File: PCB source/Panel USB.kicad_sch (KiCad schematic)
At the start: 9 parts, among them J5 Connector, USB-TYPE-C-16P, U1 PESD5V0S2BT

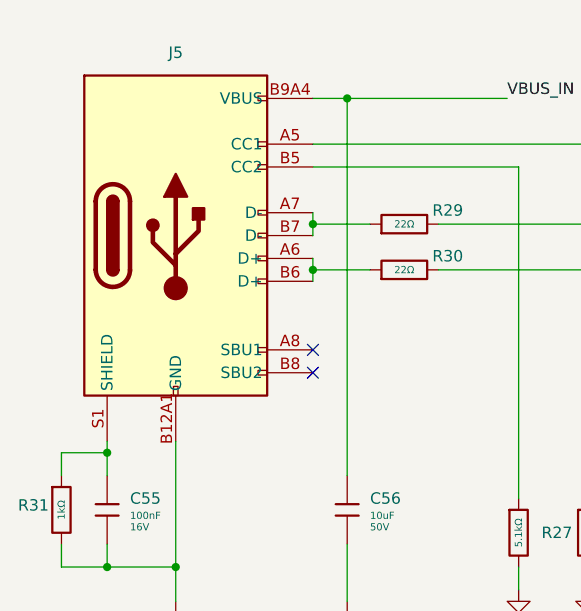
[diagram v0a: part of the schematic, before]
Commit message: Finish layout
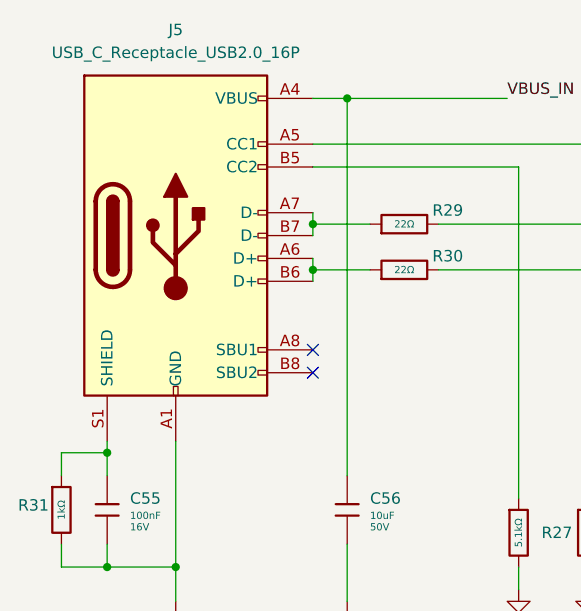
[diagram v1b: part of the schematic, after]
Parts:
- removed J5: Connector, USB-TYPE-C-16P, Connector_USB:USB_C_Receptacle_GCT_USB4105-xx-A_16P_TopMnt_Horizontal, symbol PCM_JLCPCB-Extended:Connector, USB-TYPE-C-16P
- added J5: USB_C_Receptacle_USB2.0_16P, Connector_USB:USB_C_Receptacle_GCT_USB4105-xx-A_16P_TopMnt_Horizontal, symbol Connector:USB_C_Receptacle_USB2.0_16P
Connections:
- net GND: now also J5.A1 (GND), J5.A12 (GND), J5.B1 (GND), J5.B12 (GND)
- net VBUS_IN: now also J5.A4 (VBUS), J5.A9 (VBUS), J5.B4 (VBUS), J5.B9 (VBUS)
- net at C55.1, R31.1: now also J5.S1 (SHIELD)
- net at R29.1: now also J5.A7 (D-), J5.B7 (D-)
- net at R28.1: now also J5.A5 (CC1)
- net at R30.1: now also J5.A6 (D+), J5.B6 (D+)
- net at R27.1: now also J5.B5 (CC2)
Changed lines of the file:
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@@
-	)
-	(symbol
-		(lib_id "PCM_JLCPCB-Extended:Connector, USB-TYPE-C-16P")
-		(at 96.52 85.09 0)
-		(unit 1)
-		(exclude_from_sim no)
-		(in_bom yes)
-		(on_board yes)
-		(dnp no)
-		(fields_autoplaced yes)
-		(property "Reference" "J5"
-			(at 96.52 64.77 0)
-			(effects
-				(font
-					(size 1.27 1.27)
-				)
-			)
-		)
-		(property "Value" "Connector, USB-TYPE-C-16P"
-			(at 99.06 86.36 0)
-			(effects
-				(font
-					(size 1.27 1.27)
-				)
-				(hide yes)
-			)
-		)
-		(property "Footprint" "Connector_USB:USB_C_Receptacle_GCT_USB4105-xx-A_16P_TopMnt_Horizontal"
-			(at 96.52 95.25 0)
-			(effects
-				(font
-					(size 1.27 1.27)
-					(italic yes)
-				)
-				(hide yes)
-			)
-		)
-		(property "Datasheet" "https://atta.szlcsc.com/upload/public/pdf/source/20220920/0EF8F885FCCEA71F60E9E85152155021.pdf"
-			(at 94.234 84.963 0)
-			(effects
-				(font
-					(size 1.27 1.27)
-				)
-				(justify left)
-				(hide yes)
-			)
-		)
-		(property "Description" "3A 1 Horizontal attachment 16P Female -25℃~+85℃ Type-C SMD USB Connectors ROHS"
-			(at 99.06 83.82 0)
-			(effects
-				(font
-					(size 1.27 1.27)
-				)
-				(hide yes)
-			)
-		)
-		(property "LCSC" "C2927039"
-			(at 99.06 83.82 0)
-			(effects
-				(font
-					(size 1.27 1.27)
-				)
-				(hide yes)
-			)
-		)
-		(pin "A6"
-		)
-		(pin "A12B1"
-		)
-		(pin "S1"
-		)
-		(pin "B8"
-		)
-		(pin "B12A1"
-		)
-		(pin "A9B4"
-		)
-		(pin "A7"
-		)
-		(pin "A5"
-		)
-		(pin "A8"
-		)
-		(pin "B6"
-		)
-		(pin "B7"
-		)
-		(pin "B9A4"
-		)
-		(pin "B5"
-		)
-		(instances
-			(project ""
-				(path "/3103c9de-f1ba-4d51-8bfc-798df1c75e2f/86d81324-cbad-4692-8b67-2c038a3e8215"
-					(reference "J5")
-					(unit 1)
-				)
-			)
-		)
 	)
 	(symbol
@@
 					(unit 1)
 				)
+			)
+		)
+	)
+	(symbol
+		(lib_name "USB_C_Receptacle_USB2.0_16P_1")
+		(lib_id "Connector:USB_C_Receptacle_USB2.0_16P")
+		(at 96.52 85.09 0)
+		(unit 1)
+		(exclude_from_sim no)
+		(in_bom yes)
+		(on_board yes)
+		(dnp no)
+		(fields_autoplaced yes)
+		(property "Reference" "J5"
+			(at 96.52 62.23 0)
+			(effects
+				(font
+					(size 1.27 1.27)
+				)
+			)
+		)
+		(property "Value" "USB_C_Receptacle_USB2.0_16P"
+			(at 96.52 64.77 0)
+			(effects
+				(font
+					(size 1.27 1.27)
+				)
+			)
+		)
+		(property "Footprint" "Connector_USB:USB_C_Receptacle_GCT_USB4105-xx-A_16P_TopMnt_Horizontal"
+			(at 100.33 85.09 0)
+			(effects
+				(font
+					(size 1.27 1.27)
+				)
+				(hide yes)
+			)
+		)
+		(property "Datasheet" "https://www.usb.org/sites/default/files/documents/usb_type-c.zip"
+			(at 100.33 85.09 0)
+			(effects
+				(font
+					(size 1.27 1.27)
+				)
+				(hide yes)
+			)
+		)
+		(property "Description" "USB 2.0-only 16P Type-C Receptacle connector"
+			(at 96.52 85.09 0)
+			(effects
+				(font
+					(size 1.27 1.27)
+				)
+				(hide yes)
+			)
+		)
+		(pin "A4"
+		)
+		(pin "B9"
+		)
+		(pin "A8"
+		)
+		(pin "A9"
+		)
+		(pin "B1"
+		)
+		(pin "S1"
+		)
+		(pin "A1"
+		)
+		(pin "B12"
+		)
+		(pin "A7"
+		)
+		(pin "B6"
+		)
+		(pin "B8"
+		)
+		(pin "A5"
+		)
+		(pin "A6"
+		)
+		(pin "B5"
+		)
+		(pin "B4"
+		)
+		(pin "B7"
+		)
+		(pin "A12"
+		)
+		(instances
+			(project "OrangePie"
+				(path "/3103c9de-f1ba-4d51-8bfc-798df1c75e2f/86d81324-cbad-4692-8b67-2c038a3e8215"
+					(reference "J5")
+					(unit 1)
+				)

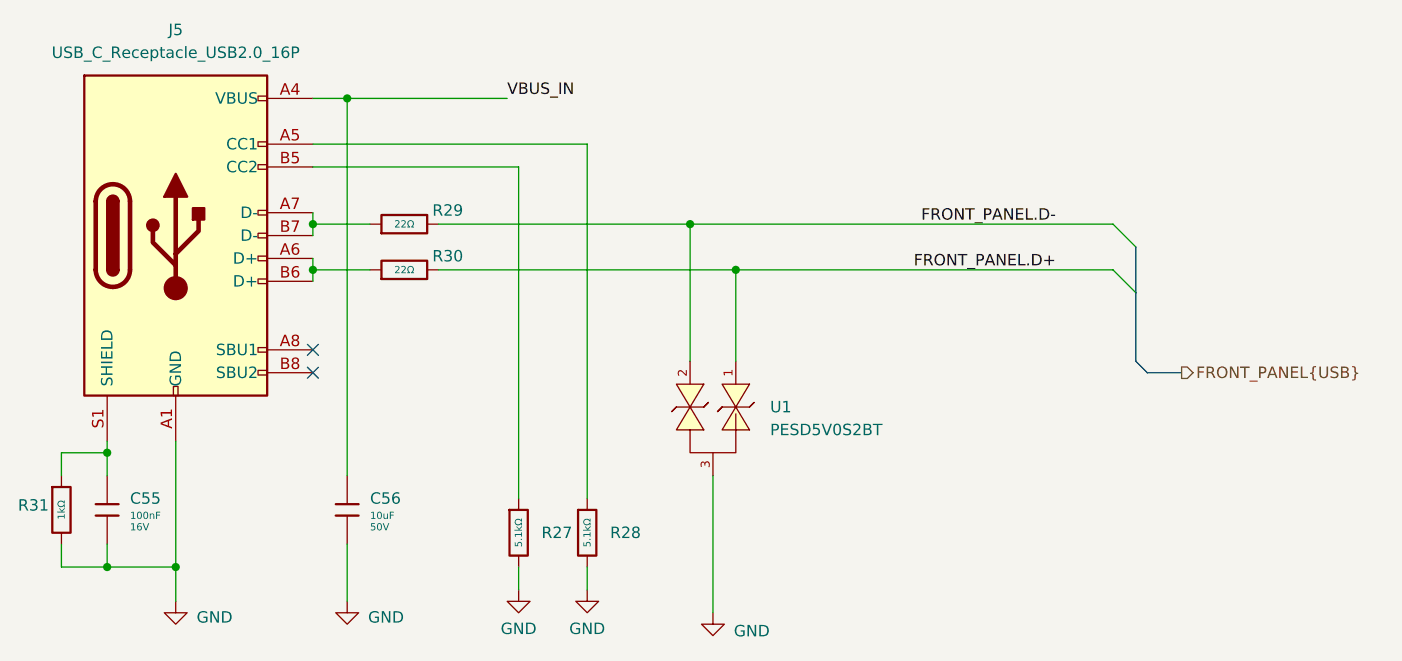
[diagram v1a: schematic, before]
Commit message: Fix schematic
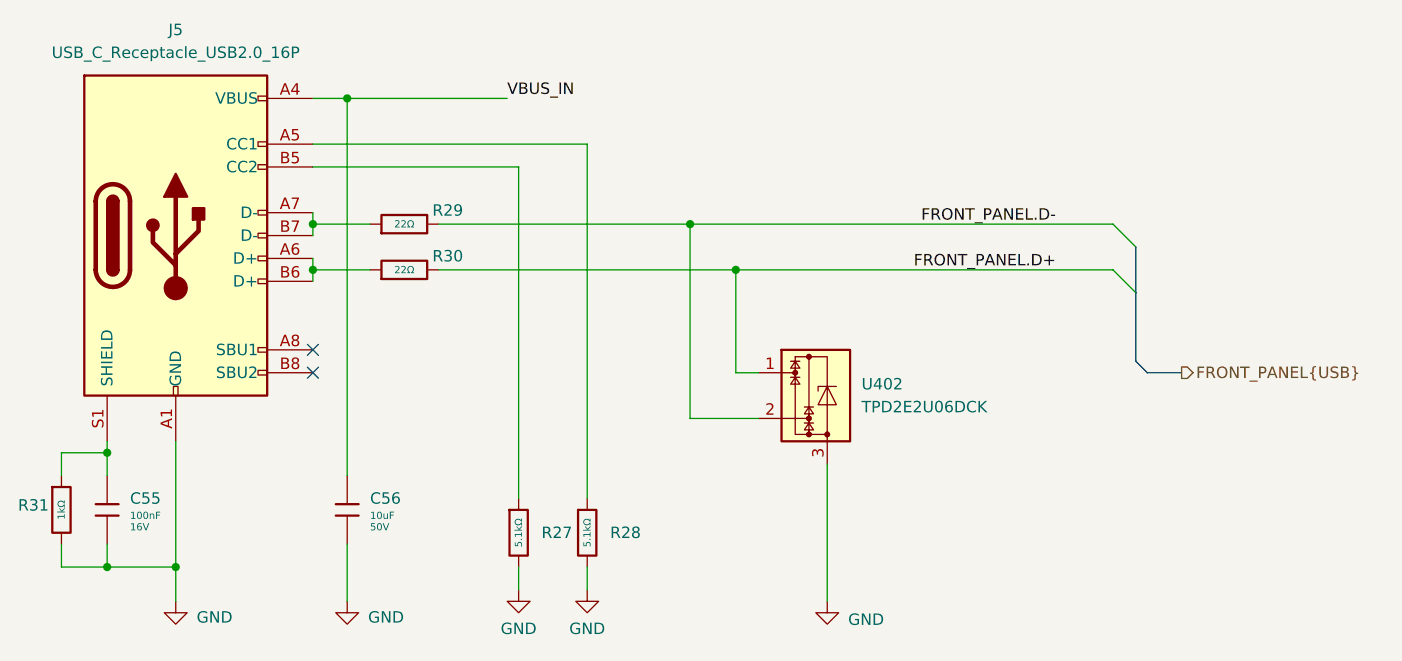
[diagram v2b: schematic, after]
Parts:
- removed U1: PESD5V0S2BT, Package_TO_SOT_SMD:SOT-23, symbol PESD5V0S2BT:PESD5V0S2BT
- added U402: TPD2E2U06DCK, Package_TO_SOT_SMD:SOT-323_SC-70, symbol Power_Protection:TPD2E2U06DCK
- C55: Stock 27771805 -> 19831671
- C56: Price 0.067USD -> 0.069USD; Stock 1423931 -> 1211974
- R27, R28: Stock 2578203 -> 3416329
- R29, R30: Stock 2497993 -> 2158519
- R31: Stock 10672962 -> 7947916
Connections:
- net FRONT_PANEL.D+: now also U402.1
- net FRONT_PANEL.D-: now also U402.2
- net GND: now also U402.3
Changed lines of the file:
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@@
 (kicad_sch
-	(version 20231120)
+	(version 20250114)
 	(generator "eeschema")
-	(generator_version "8.0")
+	(generator_version "9.0")
 	(paper "A4")
 	(title_block
@@
 		)
 	)
-	(wire
-		(pts
-			(xy 158.75 88.9) (xy 158.75 99.06)
-		)
-		(stroke
-			(width 0)
-			(type default)
-		)
-	)
-	(wire
-		(pts
-			(xy 153.67 83.82) (xy 153.67 99.06)
-		)
-		(stroke
-			(width 0)
-			(type default)
-		)
-	)
 	(bus
 		(pts
@@
 	(wire
 		(pts
+			(xy 153.67 105.41) (xy 161.29 105.41)
+		)
+		(stroke
+			(width 0)
+			(type default)
+		)
+	)
+	(wire
+		(pts
+			(xy 158.75 88.9) (xy 158.75 100.33)
+		)
+		(stroke
+			(width 0)
+			(type default)
+		)
+	)
+	(wire
+		(pts
 			(xy 111.76 88.9) (xy 111.76 90.17)
 		)
@@
 	(wire
 		(pts
-			(xy 156.21 111.76) (xy 156.21 127)
+			(xy 168.91 110.49) (xy 168.91 125.73)
 		)
 		(stroke
@@
 		(pts
 			(xy 111.76 83.82) (xy 111.76 85.09)
+		)
+		(stroke
+			(width 0)
+			(type default)
+		)
+	)
+	(wire
+		(pts
+			(xy 153.67 83.82) (xy 153.67 105.41)
+		)
+		(stroke
+			(width 0)
+			(type default)
+		)
+	)
+	(wire
+		(pts
+			(xy 158.75 100.33) (xy 161.29 100.33)
 		)
 		(stroke
@@
 	(label "FRONT_PANEL.D+"
 		(at 194.31 88.9 180)
-		(fields_autoplaced yes)
 		(effects
 			(font
@@
 	(label "FRONT_PANEL.D-"
 		(at 194.31 83.82 180)
-		(fields_autoplaced yes)
 		(effects
 			(font
@@
 	(label "VBUS_IN"
 		(at 133.35 69.85 0)
-		(fields_autoplaced yes)
 		(effects
 			(font
@@
 		(shape output)
 		(at 208.28 100.33 0)
-		(fields_autoplaced yes)
 		(effects
 			(font
@@
 			)
 		)
-		(property "Stock" "27771805"
+		(property "Stock" "19831671"
 			(at 88.9 115.57 0)
 			(effects
@@
 			)
 		)
-		(property "Stock" "2497993"
+		(property "Stock" "2158519"
 			(at 121.92 83.82 0)
 			(effects
@@
 			)
 		)
-		(property "Stock" "2578203"
+		(property "Stock" "3416329"
 			(at 142.24 118.11 0)
 			(effects
@@
 	(symbol
 		(lib_id "power:GND")
-		(at 156.21 127 0)
+		(at 168.91 125.73 0)
 		(unit 1)
 		(exclude_from_sim no)
@@
 		(dnp no)
 		(property "Reference" "#PWR0117"
-			(at 156.21 133.35 0)
+			(at 168.91 132.08 0)
 			(effects
 				(font
@@
 		)
 		(property "Value" "GND"
-			(at 160.528 129.032 0)
+			(at 173.228 127.762 0)
 			(effects
 				(font
@@
 		)
 		(property "Footprint" ""
-			(at 156.21 127 0)
+			(at 168.91 125.73 0)
 			(effects
 				(font
@@
 		)
 		(property "Datasheet" ""
-			(at 156.21 127 0)
+			(at 168.91 125.73 0)
 			(effects
 				(font
@@
 		)
 		(property "Description" "Power symbol creates a global label with name \"GND\" , ground"
-			(at 156.21 127 0)
+			(at 168.91 125.73 0)
 			(effects
 				(font
@@
 			)
 		)
-		(property "Stock" "10672962"
+		(property "Stock" "7947916"
 			(at 83.82 115.57 0)
 			(effects
@@
 				(path "/3103c9de-f1ba-4d51-8bfc-798df1c75e2f/86d81324-cbad-4692-8b67-2c038a3e8215"
 					(reference "R31")
-					(unit 1)
-				)
-			)
-		)
-	)
-	(symbol
-		(lib_id "PESD5V0S2BT:PESD5V0S2BT")
-		(at 156.21 106.68 180)
-		(unit 1)
-		(exclude_from_sim no)
-		(in_bom yes)
-		(on_board yes)
-		(dnp no)
-		(fields_autoplaced yes)
-		(property "Reference" "U1"
-			(at 162.56 104.1399 0)
-			(effects
-				(font
-					(size 1.27 1.27)
-				)
-				(justify right)
-			)
-		)
-		(property "Value" "PESD5V0S2BT"
-			(at 162.56 106.6799 0)
-			(effects
-				(font
-					(size 1.27 1.27)
-				)
-				(justify right)
-			)
-		)
-		(property "Footprint" "Package_TO_SOT_SMD:SOT-23"
-			(at 156.21 106.68 0)
-			(effects
-				(font
-					(size 1.27 1.27)
-				)
-				(hide yes)
-			)
-		)
-		(property "Datasheet" "https://www.lcsc.com/datasheet/lcsc_datasheet_2501101716_HXY-MOSFET-PESD5V0S2BT_C5451656.pdf"
-			(at 156.21 106.68 0)
-			(effects
-				(font
-					(size 1.27 1.27)
-				)
-				(hide yes)
-			)
-		)
-		(property "Description" "11A 8V 8V Bidirectional 5V SOT-23 ESD and Surge Protection (TVS/ESD)"
-			(at 156.21 106.68 0)
-			(effects
-				(font
-					(size 1.27 1.27)
-				)
-				(hide yes)
-			)
-		)
-		(pin "3"
-		)
-		(pin "1"
-		)
-		(pin "2"
-		)
-		(instances
-			(project "OrangePie"
-				(path "/3103c9de-f1ba-4d51-8bfc-798df1c75e2f/86d81324-cbad-4692-8b67-2c038a3e8215"
-					(reference "U1")
 					(unit 1)
 				)
@@
 			)
 		)
-		(property "Stock" "2497993"
+		(property "Stock" "2158519"
 			(at 121.92 88.9 0)
 			(effects
@@
 			)
 		)
-		(property "Stock" "1423931"
+		(property "Stock" "1211974"
 			(at 115.57 115.57 0)
 			(effects
@@
 			)
 		)
-		(property "Price" "0.067USD"
+		(property "Price" "0.069USD"
 			(at 115.57 115.57 0)
 			(effects
@@
 	)
 	(symbol
-		(lib_name "USB_C_Receptacle_USB2.0_16P_1")
+		(lib_id "Power_Protection:TPD2E2U06DCK")
+		(at 168.91 102.87 0)
+		(unit 1)
+		(exclude_from_sim no)
+		(in_bom yes)
+		(on_board yes)
+		(dnp no)
+		(fields_autoplaced yes)
+		(property "Reference" "U402"
+			(at 172.72 101.5999 0)
+			(effects
+				(font
+					(size 1.27 1.27)
+				)
+				(justify left)
+			)
+		)
+		(property "Value" "TPD2E2U06DCK"
+			(at 172.72 104.1399 0)
+			(effects
+				(font
+					(size 1.27 1.27)
+				)
+				(justify left)
+			)
+		)
+		(property "Footprint" "Package_TO_SOT_SMD:SOT-323_SC-70"
+			(at 148.59 109.22 0)
+			(effects
+				(font
+					(size 1.27 1.27)
+				)
+				(hide yes)
+			)
+		)
+		(property "Datasheet" "http://www.ti.com/lit/ds/symlink/tpd2e2u06.pdf"
+			(at 163.83 97.79 0)
+			(effects
+				(font
+					(size 1.27 1.27)
+				)
+				(hide yes)
+			)
+		)
+		(property "Description" "Dual-Channel High-Speed ESD Protection, SC-70"
+			(at 168.91 102.87 0)
+			(effects
+				(font
+					(size 1.27 1.27)
+				)
+				(hide yes)
+			)
+		)
+		(pin "2"
+		)
+		(pin "1"
+		)
+		(pin "3"
+		)
+		(instances
+			(project "OrangePie"
+				(path "/3103c9de-f1ba-4d51-8bfc-798df1c75e2f/86d81324-cbad-4692-8b67-2c038a3e8215"
+					(reference "U402")
+					(unit 1)
+				)
+			)
+		)
+	)
+	(symbol
 		(lib_id "Connector:USB_C_Receptacle_USB2.0_16P")
 		(at 96.52 85.09 0)
@@
 			)
 		)
-		(property "Stock" "2578203"
+		(property "Stock" "3416329"
 			(at 134.62 118.11 0)
 			(effects
